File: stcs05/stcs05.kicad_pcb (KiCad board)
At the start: 2 copper layers, 35 x 23 mm, 15 parts, among them J1 Conn_01x07_Pin, J2 Screw_Terminal_01x02, U1 STCS05DR, U2 INA169

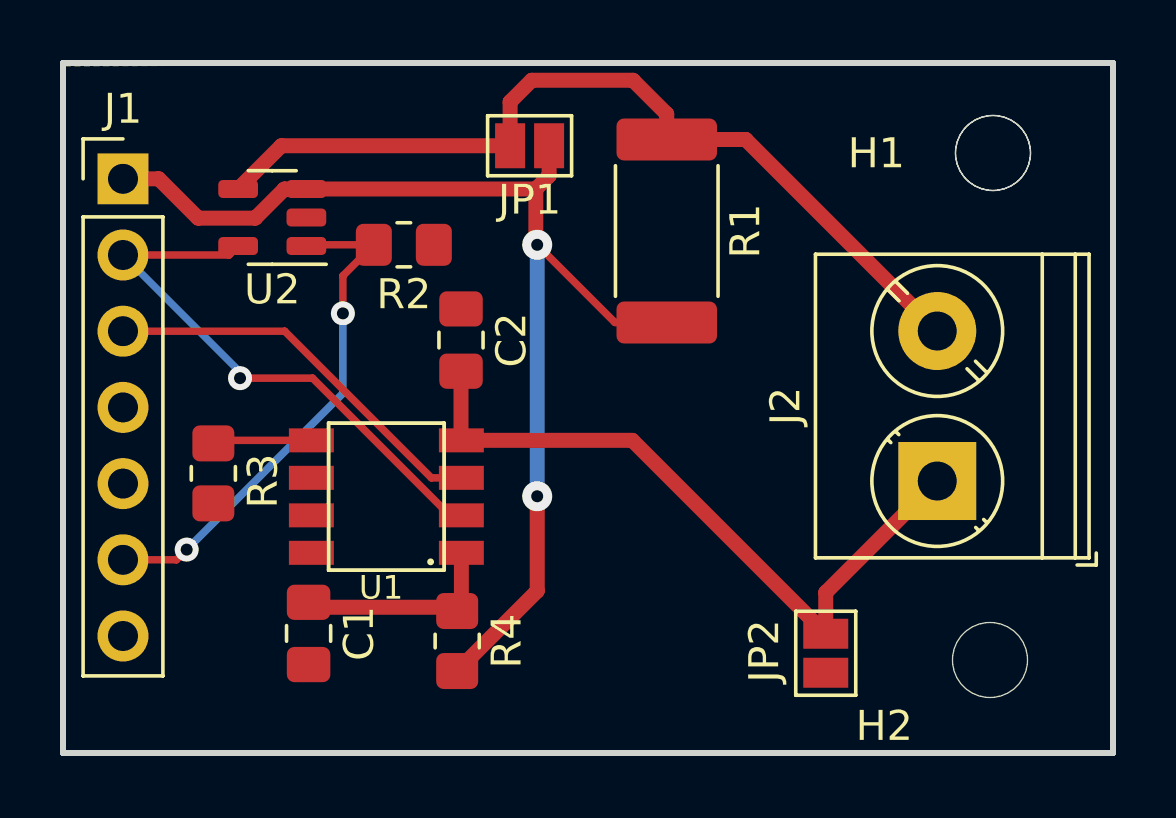
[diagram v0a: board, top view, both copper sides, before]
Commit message: ok
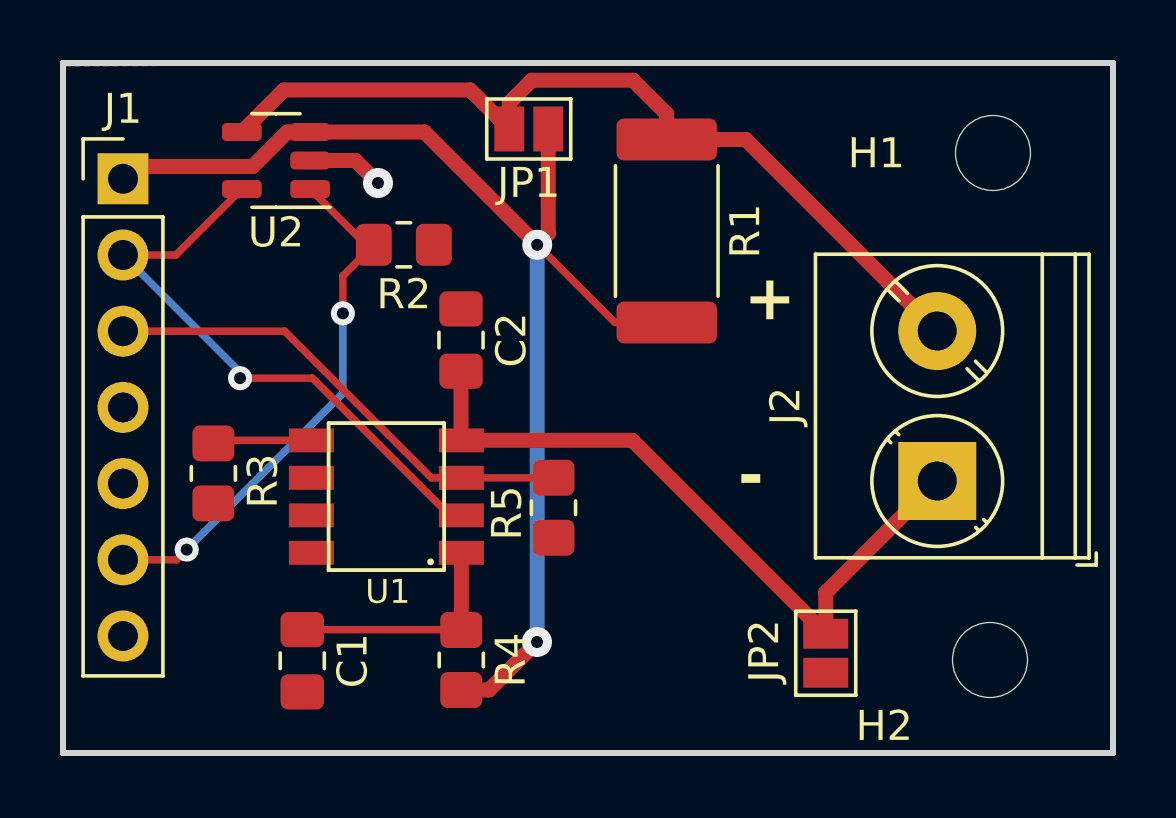
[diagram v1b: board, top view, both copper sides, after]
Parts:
- removed ?: , 
- added R5: R_Small, Resistor_SMD:R_0805_2012Metric_Pad1.20x1.40mm_HandSolder, F.Cu at (132.8, 82.4)
- moved U2 1.90 mm to (123.5, 70.8)
- moved C1 0.94 mm to (124.4, 87.5)
- moved R4 0.65 mm to (129.7, 87.5)
- moved JP1 0.56 mm to (131.9, 69.8)
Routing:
- net /I/O: track 13.3 -> 16.4 mm
- net VSS: track 38.9 -> 41.8 mm
- net GND: track 0.00 -> 2.57 mm, vias 0 -> 1
- net +3V3: track 19.0 -> 19.9 mm
- net Net-(U1-VCC): track 7.07 -> 7.88 mm
- net /ad0: track 17.3 -> 17.9 mm
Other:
- board text added: "+"
- board text added: "-"
